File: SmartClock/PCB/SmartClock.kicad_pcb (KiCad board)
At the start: 2 copper layers, 54 x 60.9 mm, 3 parts, among them SW1 SW_Push, U1 ESP32-DevKitC

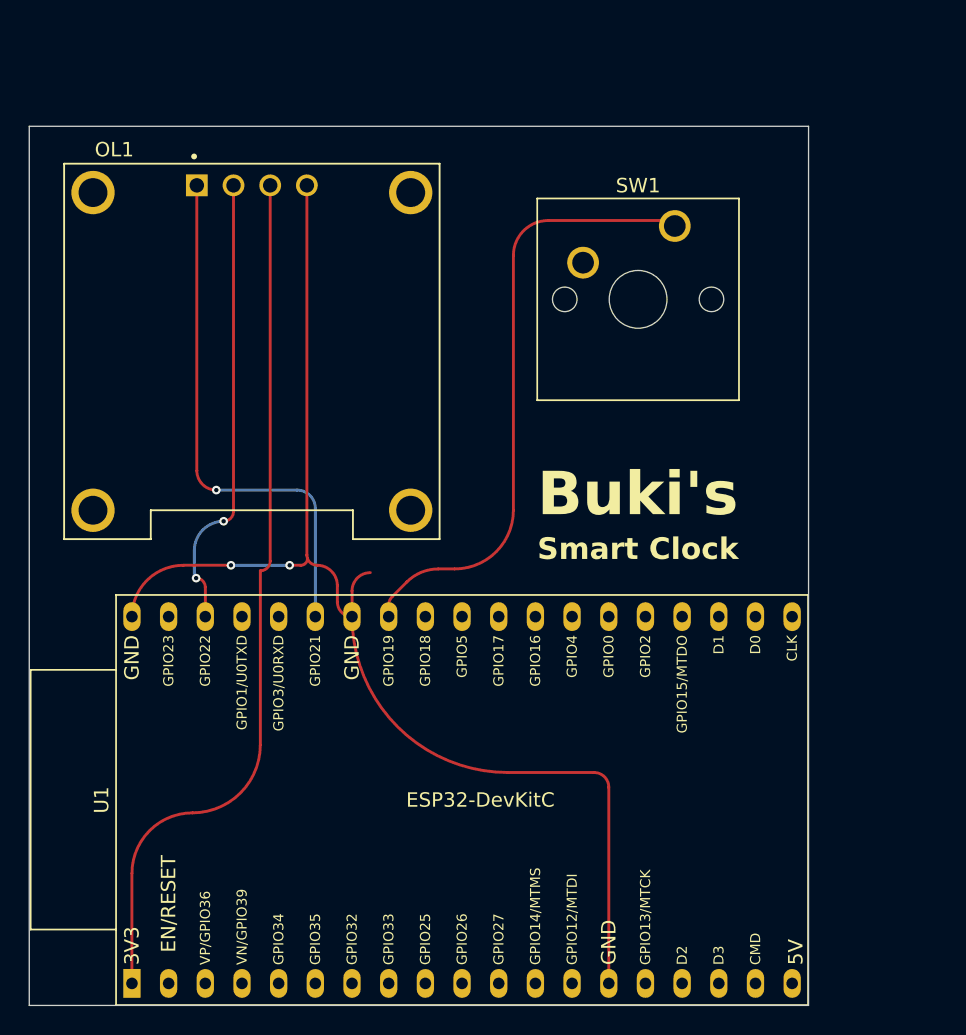
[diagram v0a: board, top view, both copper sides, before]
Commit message: changed pcb
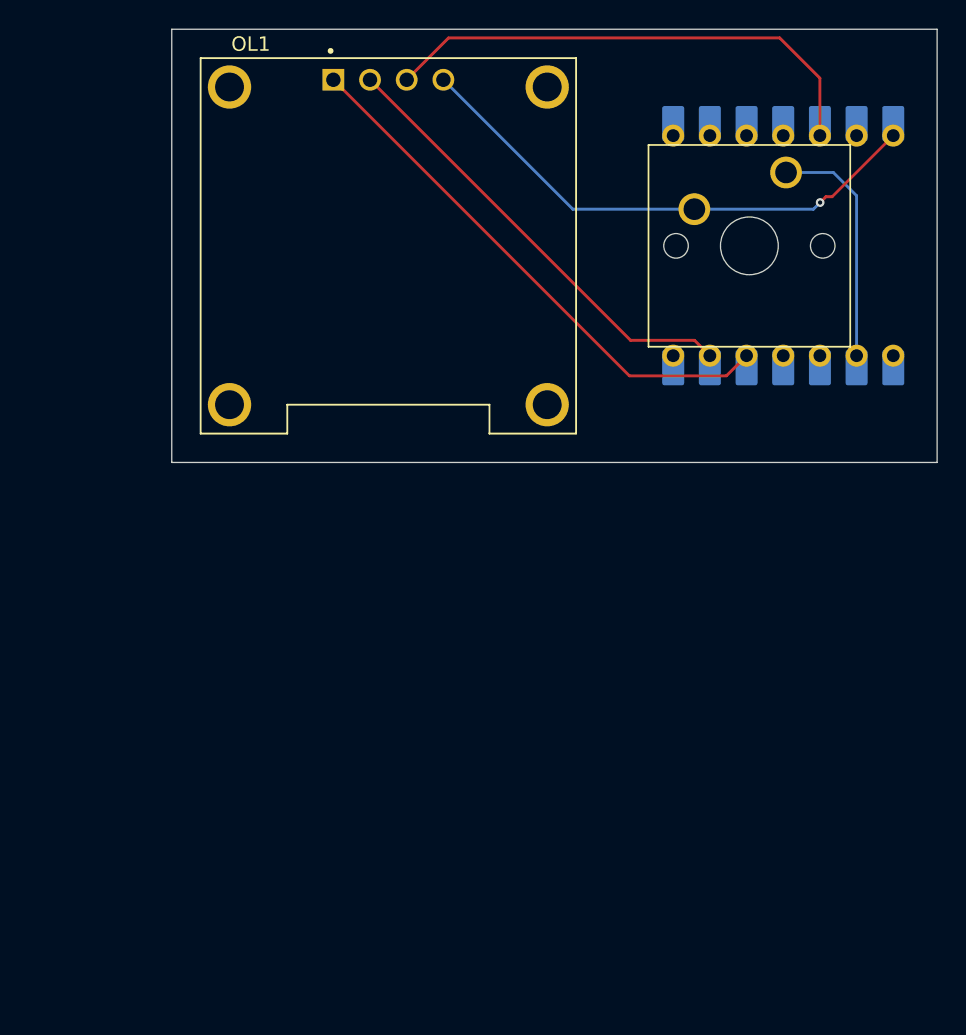
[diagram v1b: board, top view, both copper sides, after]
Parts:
- removed U1: ESP32-DevKitC, PCM_Espressif:ESP32-DevKitC
- added U2: XIAO-ESP32-C3-DIP, OPL:XIAO-ESP32-C3-DIP, B.Cu at (147.8, 49.0)
- moved OL1 11.9 mm to (120.5, 49.0)
- moved SW1 8.55 mm to (148.0, 43.9)
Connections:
- OL1 pad 4: Net-(OL1-GND) -> GND
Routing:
- net Net-(OL1-GND): track 87.2 -> 0.00 mm, vias 2 -> 0
- net GND: track 0.00 -> 37.0 mm, vias 0 -> 1
- net Net-(U2-GPIO3_A1_D1): track 43.0 -> 16.6 mm
- net Net-(OL1-VCC): track 60.3 -> 34.9 mm
- net Net-(OL1-SDA): track 36.8 -> 37.7 mm, vias 1 -> 0
- net Net-(OL1-SCL): track 31.8 -> 31.4 mm, vias 2 -> 0
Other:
- board size 54 x 60.9 mm -> 53 x 30 mm
- board text removed: "Buki's"
- board text removed: "Smart Clock"
